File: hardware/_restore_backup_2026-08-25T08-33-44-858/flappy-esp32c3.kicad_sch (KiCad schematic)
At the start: 55 parts, among them J1 USB-C-Breakout 16P, J2 LiPo 1S 500 mAh, J3 OLED SSD1306 SPI, J4 Arcade-Taster, SW1 Ein/Aus, U1 ESP32-C3-WROOM-02-N4, U2 MCP73831-2-OT, U3 AP2112K-3.3

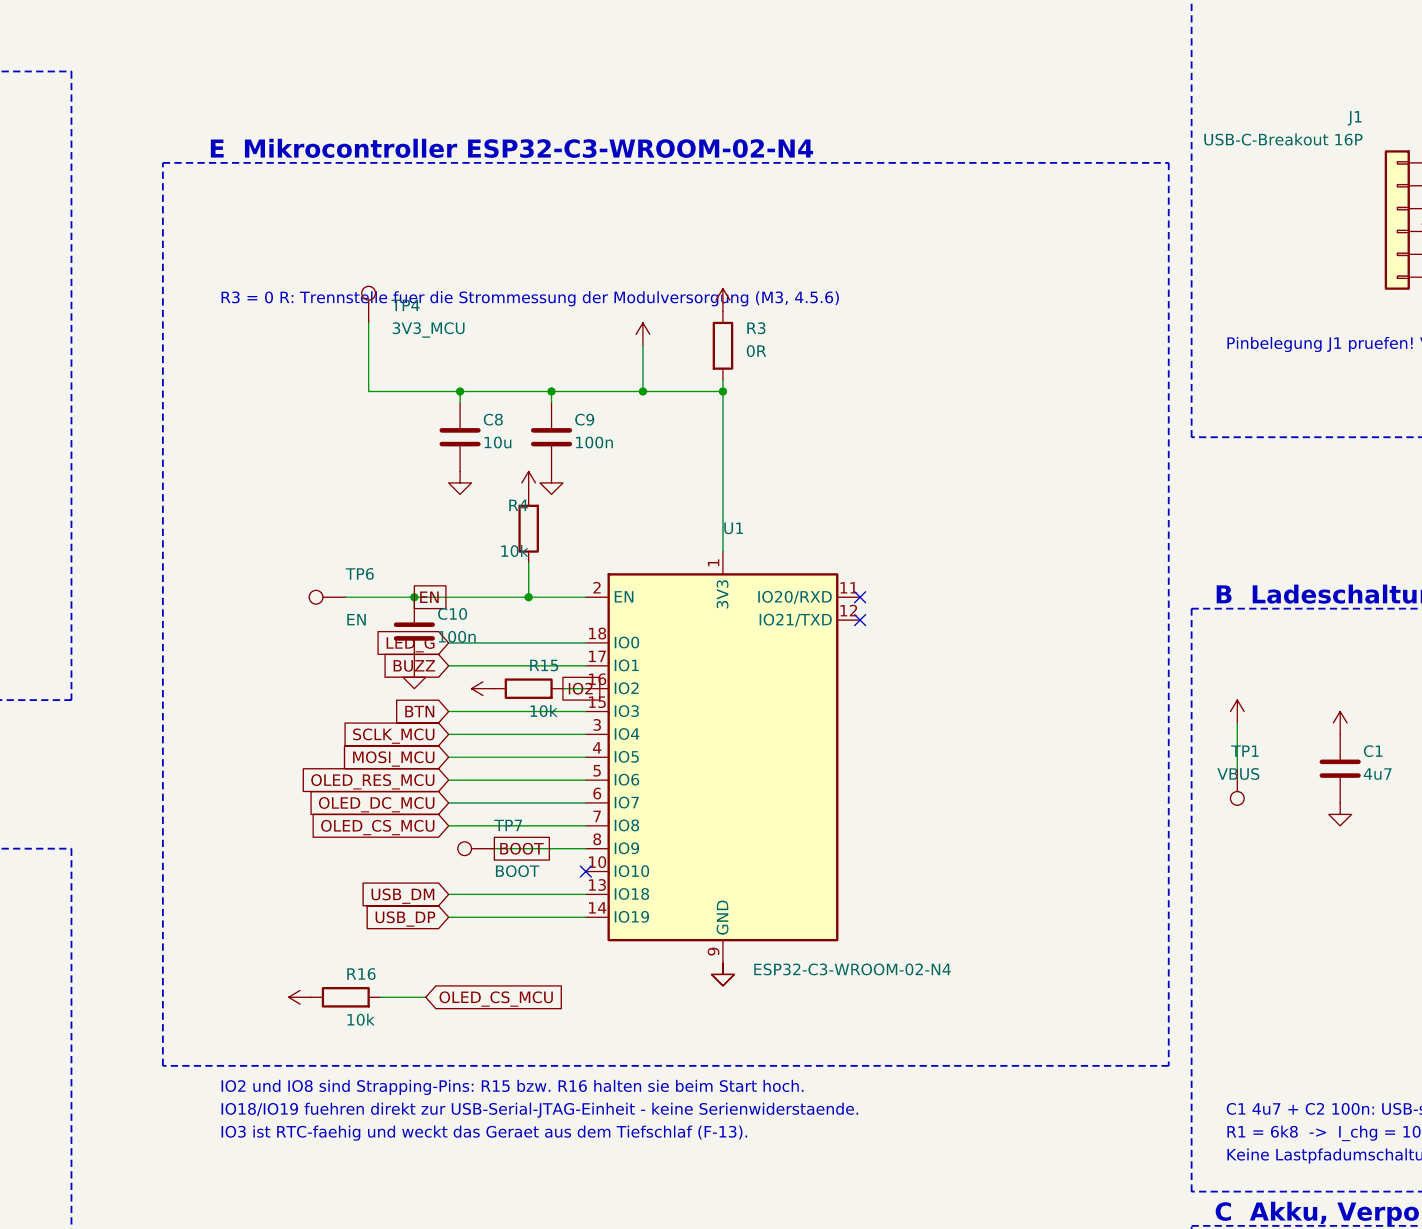
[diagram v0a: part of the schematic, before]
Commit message: .
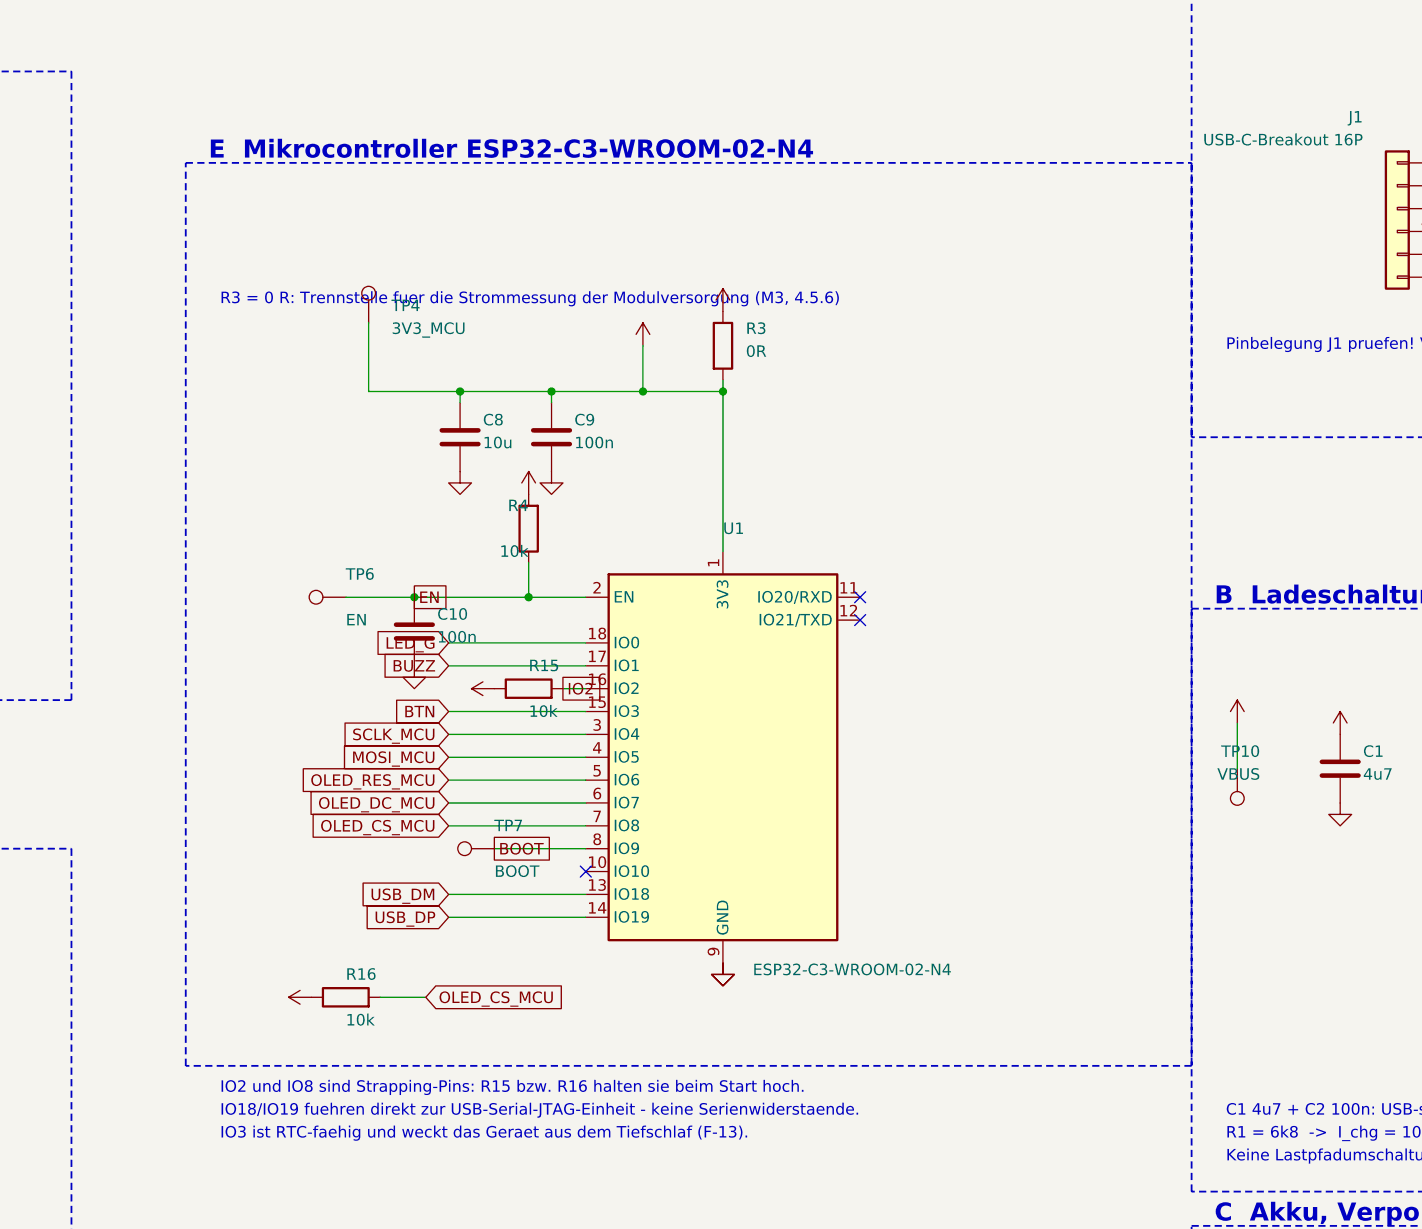
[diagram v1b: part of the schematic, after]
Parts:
- renumbered TP1 to TP10
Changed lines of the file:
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@@
 	)
 	(rectangle
-		(start 182.88 40.64)
-		(end 294.64 140.97)
+		(start 185.42 40.64)
+		(end 297.18 140.97)
 		(stroke
 			(width 0.2)
@@
 		(dnp no)
 		(fields_autoplaced yes)
-		(property "Reference" "TP1"
+		(property "Reference" "TP10"
 			(at 304.8 106.045 0)
 			(show_name no)
@@
 			(project "flappy-esp32c3"
 				(path "/ccaf1aec-7edc-5c5d-bbbd-2f38978655ed"
-					(reference "TP1")
+					(reference "TP10")
 					(unit 1)
 				)
